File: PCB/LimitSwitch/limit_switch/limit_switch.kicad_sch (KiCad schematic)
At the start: 15 parts, among them J1 Conn_01x03_Pin, J2 Conn_01x03_Pin, T1 Transformer_1P_1S, U1 LM358

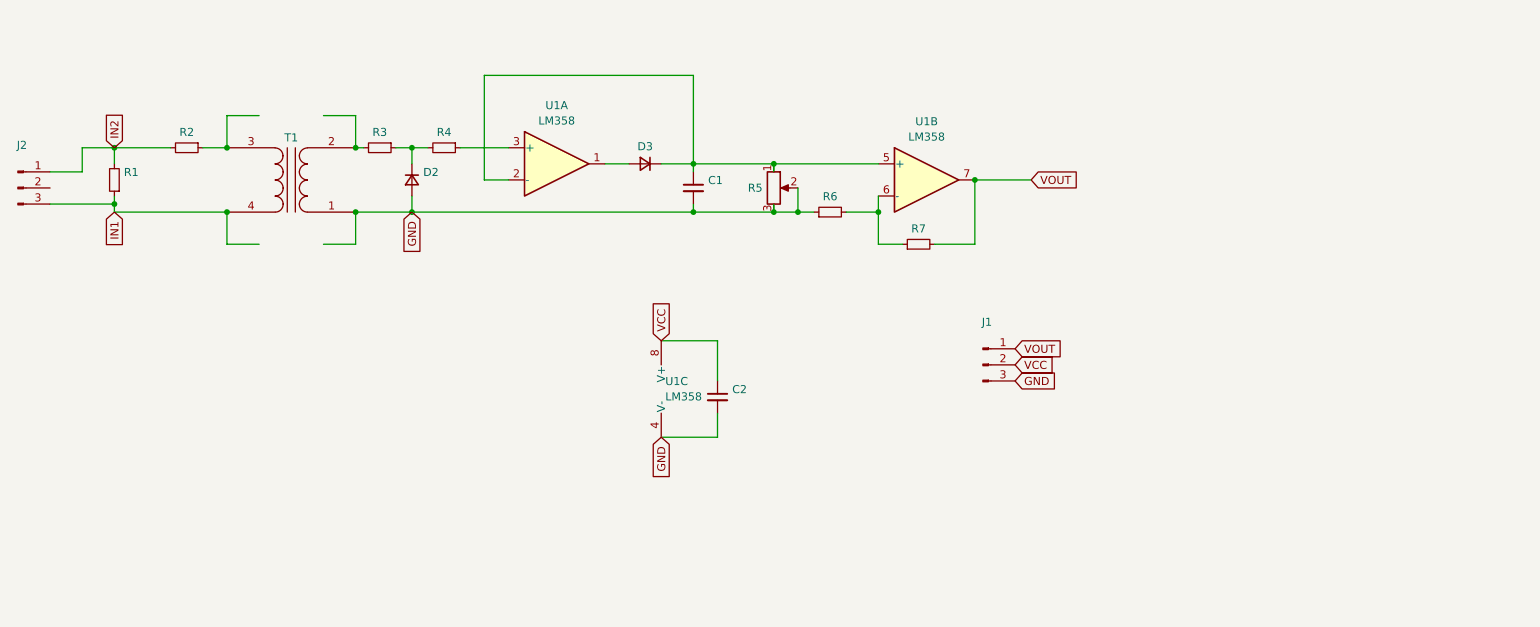
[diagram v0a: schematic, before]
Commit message: 5
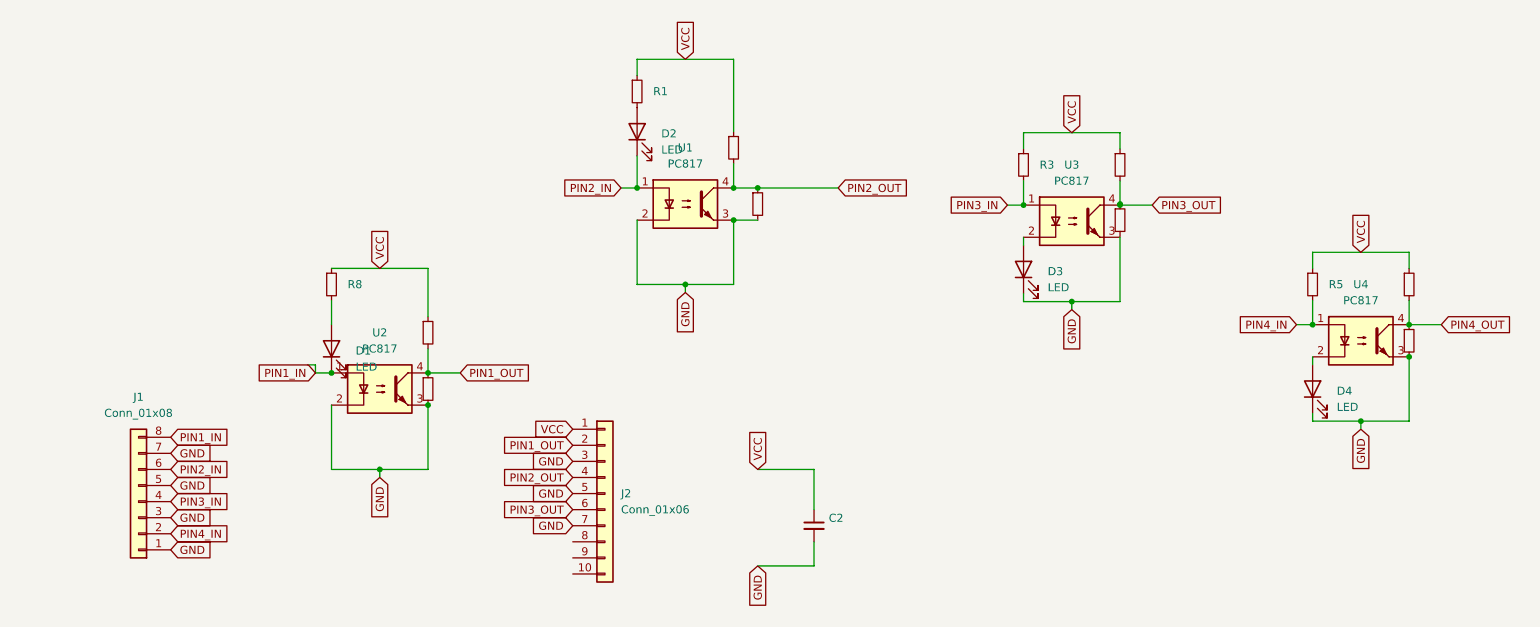
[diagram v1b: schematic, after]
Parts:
- removed C1: C_Small, Capacitor_SMD:C_1206_3216Metric_Pad1.33x1.80mm_HandSolder, symbol Device:C_Small
- removed D2, D3: D_Small, Diode_SMD:D_MicroMELF_Handsoldering, symbol Device:D_Small
- removed J1, J2: Conn_01x03_Pin, Connector_PinHeader_2.54mm:PinHeader_1x03_P2.54mm_Vertical, symbol Connector:Conn_01x03_Pin
- removed R5: R_Small, Potentiometer_THT:Potentiometer_Bourns_3266Y_Vertical, symbol Device:R_Potentiometer
- removed T1: Transformer_1P_1S, Transformer_THT:Transformer_Zeming_ZMPT101K, symbol Device:Transformer_1P_1S
- removed U1: LM358, Package_SO:SO-8_3.9x4.9mm_P1.27mm, symbol Amplifier_Operational:LM358
- added D1, D2, D3, D4: LED, Resistor_SMD:R_0805_2012Metric_Pad1.20x1.40mm_HandSolder, symbol Device:LED
- added J1: Conn_01x08, Connector_PinHeader_2.54mm:PinHeader_1x08_P2.54mm_Vertical, symbol Connector_Generic:Conn_01x08
- added J2: Conn_01x06, Connector_PinHeader_2.54mm:PinHeader_1x09_P2.54mm_Vertical, symbol Connector_Generic:Conn_01x10
- added R10, R11, R12, R5, R8, R9: R_Small, Resistor_SMD:R_1206_3216Metric_Pad1.30x1.75mm_HandSolder, symbol Device:R_Small
- added U1, U2, U3, U4: PC817, Package_DIP:DIP-4_W8.89mm_SMDSocket_LongPads, symbol Isolator:PC817
- R1: footprint Resistor_SMD:R_2512_6332Metric_Pad1.40x3.35mm_HandSolder -> Resistor_SMD:R_1206_3216Metric_Pad1.30x1.75mm_HandSolder
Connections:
- net IN1 is gone; now on net VCC: R1.1
- net VOUT is gone; now on net GND: R7.2
- net GND: now also D3.1 (K), D4.1 (K), J1.1 (Pin_1), J1.3 (Pin_3), J1.5 (Pin_5), J1.7 (Pin_7), J2.3 (Pin_3), J2.5 (Pin_5), J2.7 (Pin_7), R11.2, R12.2, U1.2, U1.3, U2.2, U2.3, U3.3, U4.3; no longer R6.1
- net VCC: now also R2.1, R3.1, R4.1, R6.1, J2.1 (Pin_1), R5.1, R8.1, R9.1
- net PIN2_OUT: now reaches R7.1
- net PIN2_OUT: now also R2.2, J2.4 (Pin_4), U1.4; no longer R6.2
- net PIN3_OUT: now reaches R4.2
- net PIN3_OUT: now also J2.6 (Pin_6), R10.1, U3.4; no longer R3.1
- net PIN3_IN: now reaches R3.2
- net PIN3_IN: now also J1.4 (Pin_4), U3.1
- net IN2: no longer names the net of R1.2
- net IN2: now also D2.2 (A); no longer R2.2
- new net: D1.2 (A), R8.2
- new net: D4.2 (A), U4.2
- new net: D3.2 (A), U3.2
- new net PIN1_IN: D1.1 (K), J1.8 (Pin_8), U2.1
- new net PIN1_OUT: J2.2 (Pin_2), R12.1, R9.2, U2.4
- new net PIN2_IN: D2.1 (K), J1.6 (Pin_6), U1.1
- new net PIN4_IN: J1.2 (Pin_2), R5.2, U4.1
- new net PIN4_OUT: R11.1, R6.2, U4.4
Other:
- moved on the sheet: C2
